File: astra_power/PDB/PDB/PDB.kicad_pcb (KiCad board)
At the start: 2 copper layers, 125.5 x 91 mm, 6 parts, among them J1 Screw_Terminal_01x02, J2 Screw_Terminal_01x10, J3 Screw_Terminal_01x10, J4 Screw_Terminal_01x02

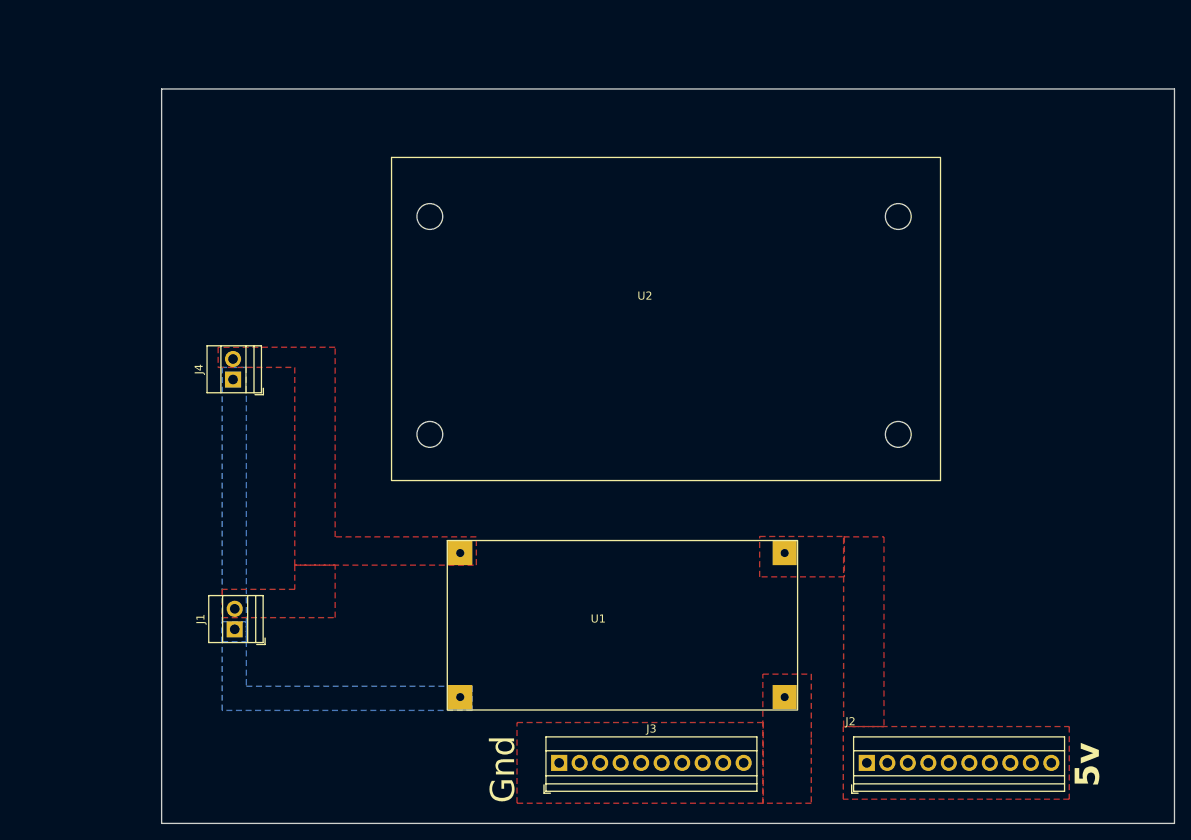
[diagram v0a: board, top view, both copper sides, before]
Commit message: uploaded PDB
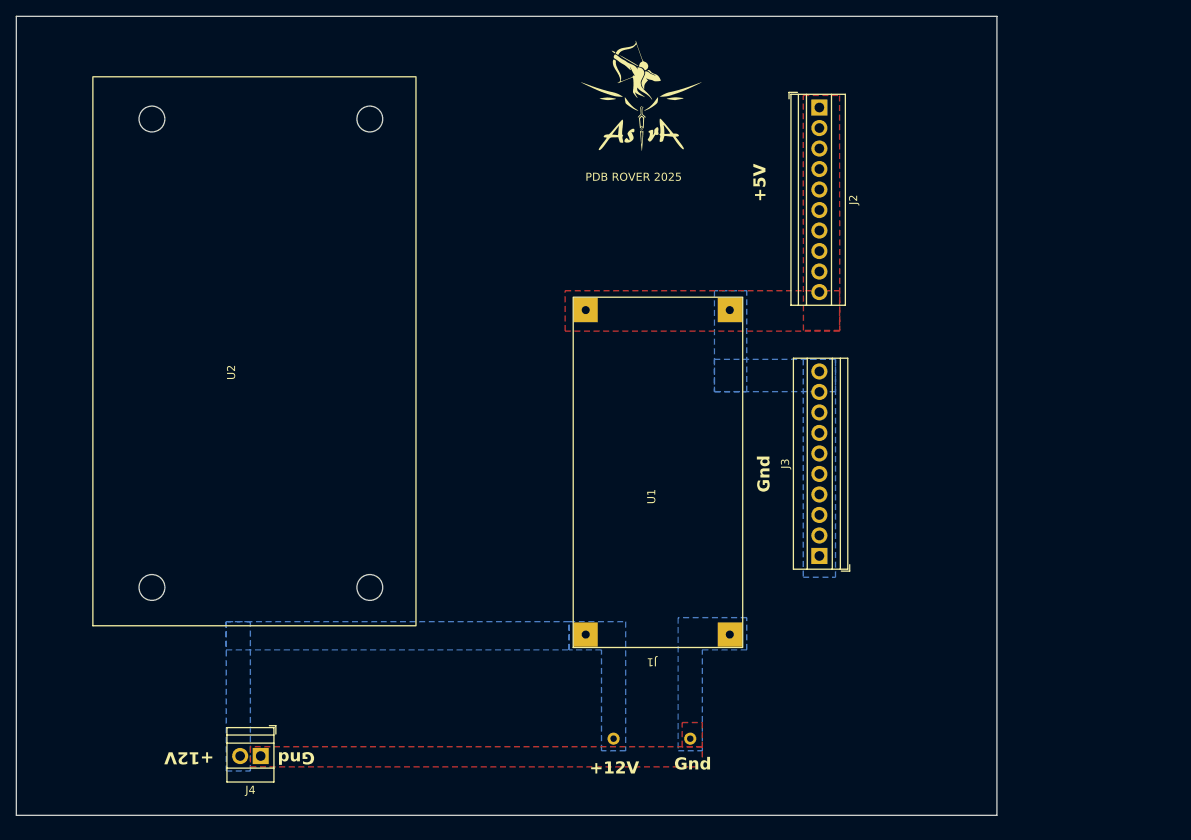
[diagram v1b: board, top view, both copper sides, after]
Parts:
- added G***: LOGO, LOGO, F.Cu at (153.0, 64.5)
- J1: footprint TerminalBlock:TerminalBlock_Xinya_XY308-2.54-2P_1x02_P2.54mm_Horizontal -> custom_terminal:Barrier pins
- moved J2 81.4 mm to (175.0, 65.3), turned to -90 degrees
- moved J1 53.4 mm to (154.2, 143.5), turned to 180 degrees
- moved J4 46.8 mm to (105.8, 145.7), turned to 180 degrees
- moved J3 41.2 mm to (175.0, 120.9), turned to 90 degrees
- moved U2 34.8 mm to (107.9, 119.0), turned to 90 degrees
- moved U1 34.3 mm to (163.9, 130.6), turned to 90 degrees
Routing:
- added copper zone on B.Cu, net Vin+
- added copper zone on F.Cu, net vin-
- added copper zone on B.Cu, net vout-
- removed copper zone on F.Cu, net Vin+
- removed copper zone on F.Cu, net vout-
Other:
- board size 125.5 x 91 mm -> 121.5 x 99 mm
- board text added: "+12V"
- board text added: "+5V"
- board text added: "PDB ROVER 2025"
- board text removed: "5v"
